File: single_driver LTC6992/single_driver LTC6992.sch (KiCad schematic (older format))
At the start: 39 parts, among them J1 Conn_02x02_Counter_Clockwise, J2 Screw_Terminal_01x02, J3 Conn_01x08_Male, SW1 SW_DIP_x06, U1 LTC6992-1 (Rev. D), U2 LM7805_TO220, U3 DRV10970

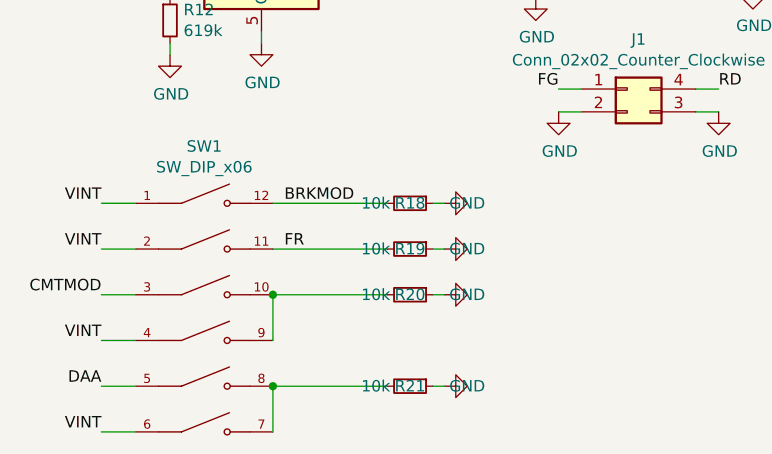
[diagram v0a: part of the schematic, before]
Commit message: Basically finished pcb
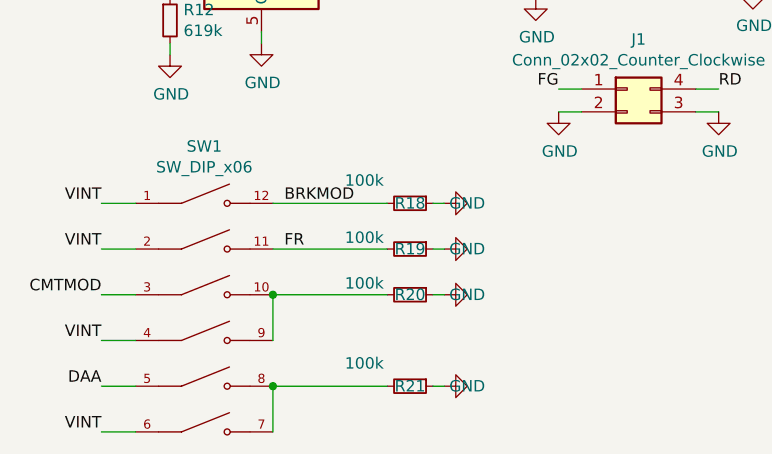
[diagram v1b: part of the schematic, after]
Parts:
- R18, R19, R20, R21: value 10k -> 100k
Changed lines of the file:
@@
 P 4250 5350
 F 0 "R20" V 4250 5350 50  0000 C CNN
-F 1 "10k" V 4250 5200 50  0000 C CNN
+F 1 "100k" V 4200 5150 50  0000 C CNN
 F 2 "Resistor_SMD:R_0603_1608Metric" H 4250 5350 50  0001 C CNN
 F 3 "~" H 4250 5350 50  0001 C CNN
@@
 P 4250 4950
 F 0 "R18" V 4250 4950 50  0000 C CNN
-F 1 "10k" V 4250 4800 50  0000 C CNN
+F 1 "100k" V 4150 4750 50  0000 C CNN
 F 2 "Resistor_SMD:R_0603_1608Metric" H 4250 4950 50  0001 C CNN
 F 3 "~" H 4250 4950 50  0001 C CNN
@@
 P 4250 5150
 F 0 "R19" V 4250 5150 50  0000 C CNN
-F 1 "10k" V 4250 5000 50  0000 C CNN
+F 1 "100k" V 4200 4950 50  0000 C CNN
 F 2 "Resistor_SMD:R_0603_1608Metric" H 4250 5150 50  0001 C CNN
 F 3 "~" H 4250 5150 50  0001 C CNN
@@
 P 4250 5750
 F 0 "R21" V 4250 5750 50  0000 C CNN
-F 1 "10k" V 4250 5600 50  0000 C CNN
+F 1 "100k" V 4150 5550 50  0000 C CNN
 F 2 "Resistor_SMD:R_0603_1608Metric" H 4250 5750 50  0001 C CNN
 F 3 "~" H 4250 5750 50  0001 C CNN
